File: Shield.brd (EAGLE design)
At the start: 53.3 x 58.4 mm, 18 parts, among them Q8 TIP120, U2 ARDUINO_SHIELDNO_SILK

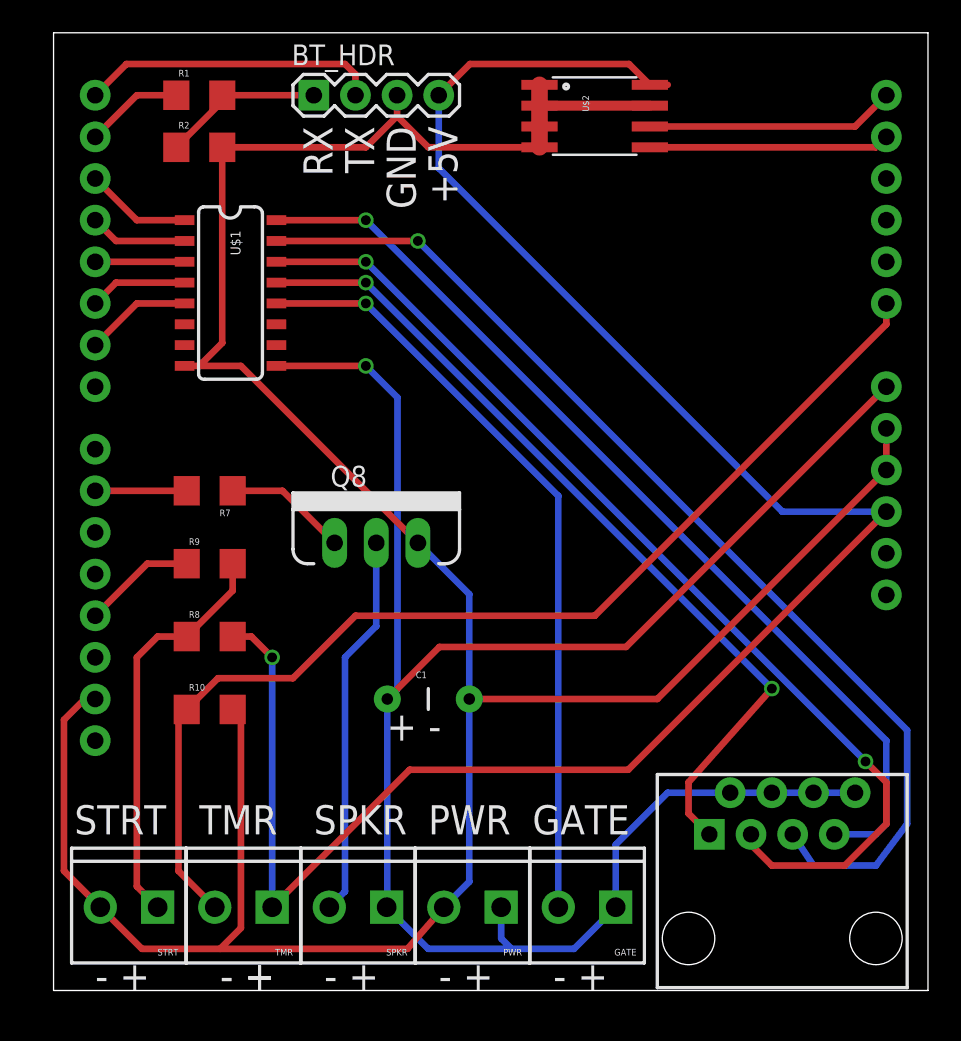
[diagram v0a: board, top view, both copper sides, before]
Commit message: Converted to single board
git-svn-id: svn+ssh://petrocik.net/home/svn/repo/uci_gate/branches/hardware/uci_gate/3.x@90 8c868176-b666-4d83-8e7f-acb7c29fc81a
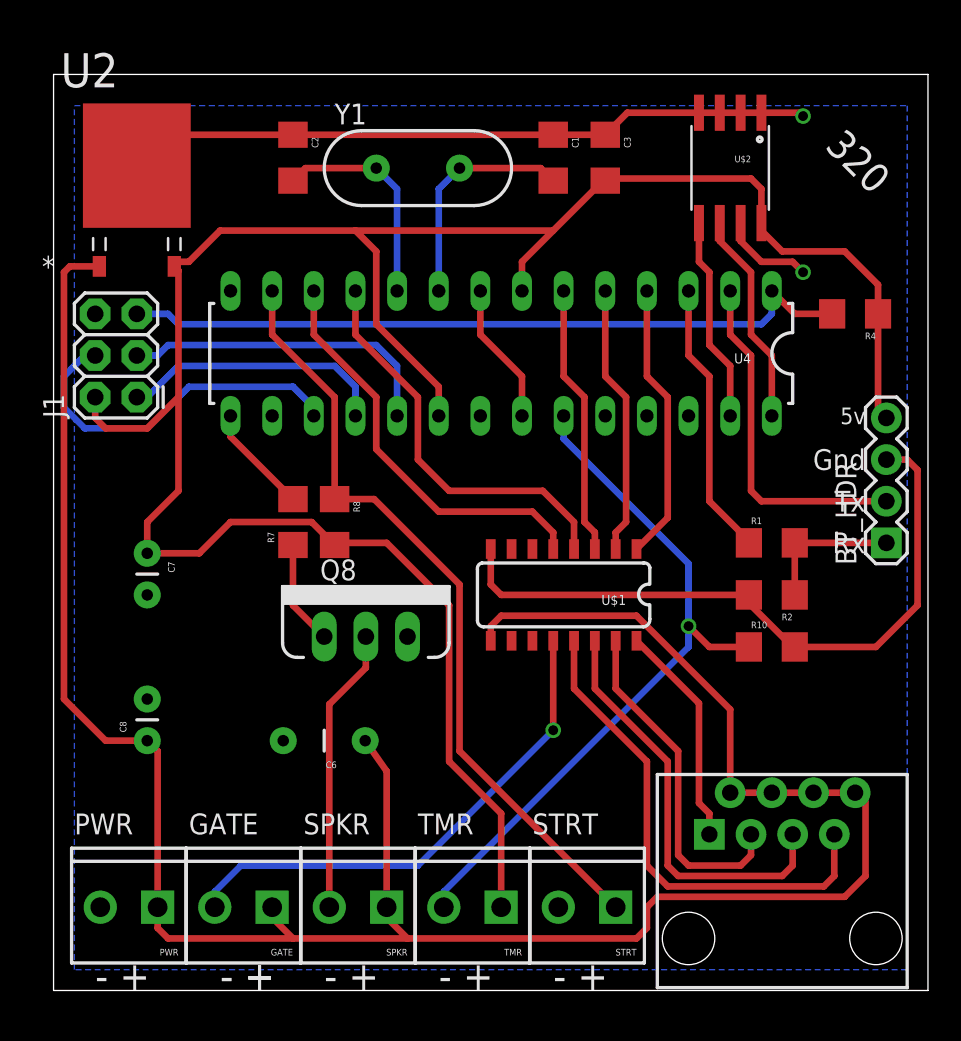
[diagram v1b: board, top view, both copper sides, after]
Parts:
- removed R9: 100, SparkFun-Passives:1206
- added C2: 22pf, SparkFun-Capacitors:1206
- added C3: 0.1uf, SparkFun-Capacitors:1206
- added C6: (no value), SparkFun-Capacitors:CAP-PTH-5MM
- added C7, C8: 10uf, SparkFun-Capacitors:CAP-PTH-SMALL
- added J1: AVR_SPI_PRG_6PTH, SparkFun-Connectors:2X3
- added R4: 10K, SparkFun-Passives:1206
- added U4: ATMEGA328P_PDIP, SparkFun-DigitalIC:DIL28-3
- added Y1: 16Mhz, SparkFun-FreqCtrl:HC49US
- C1: value (none) -> 22pf; device SparkFun-Capacitors:CAP-PTH-5MM -> SparkFun-Capacitors:1206
- U2: value ARDUINO_SHIELDNO_SILK -> LM78XX-TO252-3; device SparkFun-Boards:DUEMILANOVE_VIAS -> element14-com:TO252-3
- moved BT_HDR 44.3 mm to (50.8, 27.3), turned to 90 degrees
- moved R1 44.3 mm to (43.8, 27.3)
- moved R2 44.3 mm to (43.8, 24.1), turned to 180 degrees
- moved U2 37.8 mm to (5.08, 50.2)
- moved R10 34.5 mm to (43.8, 21.0)
- moved C1 33.9 mm to (30.5, 50.8), turned to 270 degrees
- moved STRT 27.9 mm to (34.3, 5.08)
- moved U$1 27.4 mm to (31.1, 24.1), turned to 180 degrees
- moved GATE 21.0 mm to (13.3, 5.08)
- moved PWR 21.0 mm to (6.35, 5.08)
- moved TMR 14.0 mm to (27.3, 5.08)
- moved R8 10.3 mm to (17.1, 28.6), turned to 270 degrees
- moved U$2 8.84 mm to (41.3, 50.2), turned to 180 degrees
- moved Q8 5.75 mm to (19.1, 21.6)
- moved R7 5.43 mm to (14.6, 28.6), turned to 90 degrees
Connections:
- net N$6 renamed GATE
- removed net N$1 (its old number): U$1.1, U2.D2
- removed net N$10: LIGHT.7, U$1.16
- removed net N$11: U$2.6, U2.A5
- removed net N$13: R7.2, U2.D9
- removed net N$14: U$2.5, U2.A4
- removed net N$16: BT_HDR.2, U2.RX
- removed net N$18: BT_HDR.4, R8.2, TMR.1, U$2.8, U2.5V
- removed net N$20: R9.1, U2.D12
- removed net N$21: R8.1, R9.2, STRT.1
- removed net N$22: R10.1, TMR.2, U2.A0
- removed net N$23: R1.1, U2.TX
- removed net N$7: LIGHT.1, U$1.13
- removed net N$8: LIGHT.3, U$1.14
- removed net N$9: LIGHT.5, U$1.15
- new net 5V: BT_HDR.4, C3.2, C7.1, J1.2, R4.1, R8.2, TMR.1, U$2.8, U2.3, U4.20, U4.7
- new net A0: R10.1, TMR.2, U4.23
- new net A4: U$2.5, U4.27
- new net A5: U$2.6, U4.28
- new net D2: U$1.1, U4.4
- new net D3: U$1.2, U4.5
- new net D4: U$1.3, U4.6
- new net D5: U$1.4, U4.11
- new net D6: U$1.5, U4.12
- new net D7: R8.1, STRT.1, U4.13
- new net D9: R7.2, U4.15
- new net MISO: J1.1, U4.18
- new net MOSI: J1.4, U4.17
- new net N$15: C1.2, U4.9, Y1.2
- new net N$24: C2.2, U4.10, Y1.1
- new net RESET: J1.5, R4.2, U4.1
- new net RX: BT_HDR.2, U4.2
- new net SCK: J1.3, U4.19
- new net TX: R1.1, U4.3
- net GND: now also C1.1, C2.1, C3.1, C6.2, C7.2, C8.2, J1.6, U2.2, U4.22, U4.8; no longer C1.2, U2.GND@0, U2.GND@1, U2.GND@2
- net N$2: now also LIGHT.1, U$1.16; no longer U$1.2, U2.D3
- net N$3: now also LIGHT.3, U$1.15; no longer U$1.3, U2.D4
- net N$4: now also LIGHT.5, U$1.14; no longer U$1.4, U2.D5
- net N$5: now also LIGHT.7, U$1.13; no longer U$1.5, U2.D6
- net VCC: now also C6.1, C8.1, U2.1; no longer C1.1, U2.VIN
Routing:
- net 5V: track 0.00 -> 142.5 mm
- net N$18: track 121.4 -> 0.00 mm, vias 1 -> 0
- net GND: track 177.0 -> 99.1 mm, vias 0 -> 2
- net N$22: track 67.2 -> 0.00 mm
- net N$9: track 65.8 -> 0.00 mm, vias 1 -> 0
- net N$8: track 63.4 -> 0.00 mm, vias 2 -> 0
- net N$10: track 58.9 -> 0.00 mm, vias 1 -> 0
- net N$7: track 51.8 -> 0.00 mm, vias 2 -> 0
- net D7: track 0.00 -> 47.7 mm
- net RESET: track 0.00 -> 44.9 mm
- net A0: track 0.00 -> 43.5 mm, vias 0 -> 1
- net VCC: track 116.5 -> 143.9 mm, vias 1 -> 0
- net D6: track 0.00 -> 25.1 mm
- net N$21: track 24.9 -> 0.00 mm
- net D5: track 0.00 -> 24.6 mm
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- added copper zone on layer 16, net GND
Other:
- board size 53.3 x 58.4 mm -> 53.3 x 55.9 mm
- board text added: "320"
- board text added: "5v"
- board text added: "Gnd"
- board text added: "Rx"
- board text added: "Tx"
- board text added: "UCI Gate v3.0"
- board text removed: "+ -"
- board text removed: "+5V"
- board text removed: "GND"
- board text removed: "RX"
- board text removed: "TX"
- board text removed: "UCI Gate v2.3"
